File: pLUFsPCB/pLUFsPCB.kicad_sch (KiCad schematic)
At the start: 9 parts, among them J1 Circular Display Pins (R), J2 Circular Display Pins (L), M1 Stepper_Motor_bipolar, SW2 BT Button, U1 ESP32 C3, U2 TB6612FNG

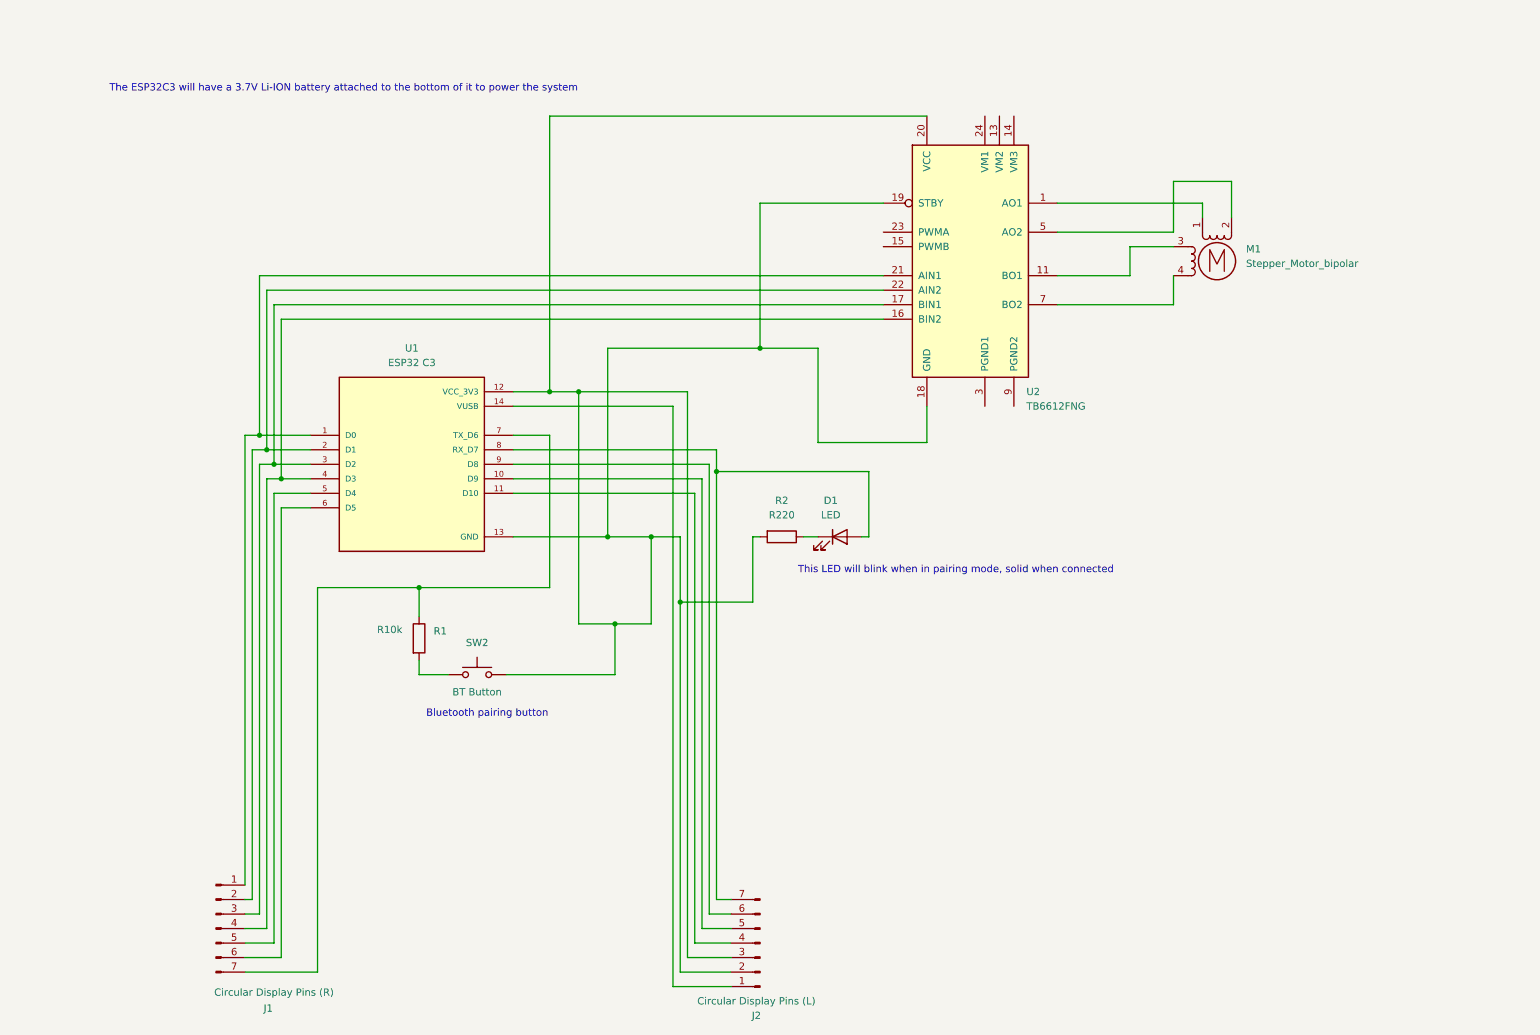
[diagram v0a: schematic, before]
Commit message: lots
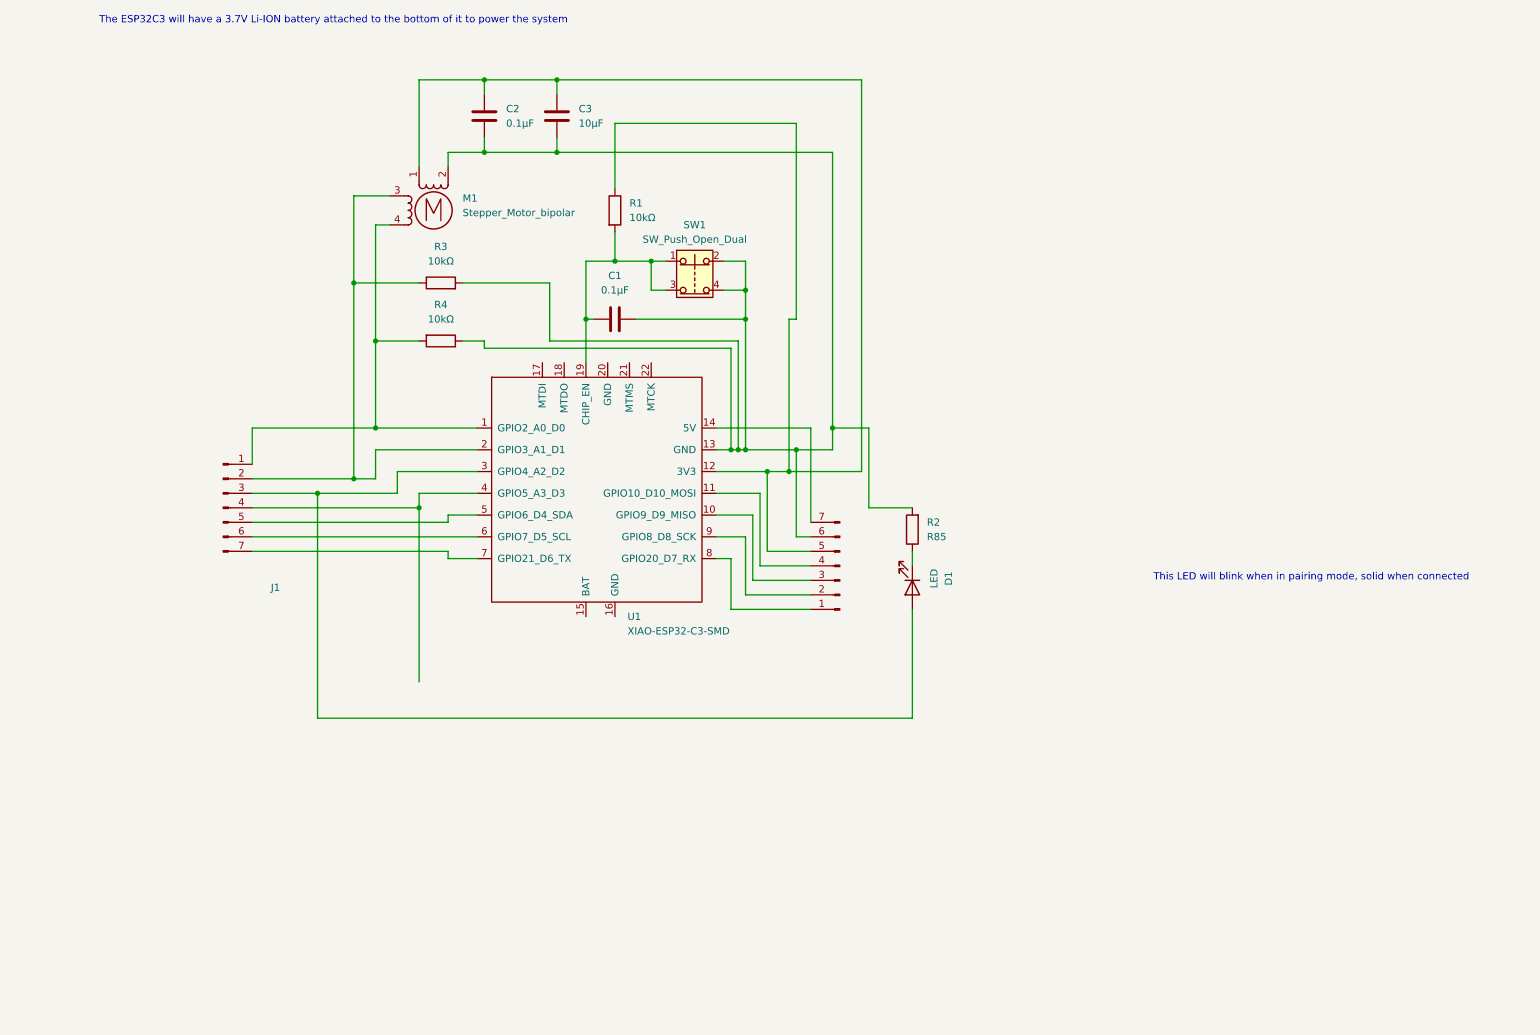
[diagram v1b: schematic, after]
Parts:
- removed SW2: BT Button, symbol Switch:SW_Push
- removed U1: ESP32 C3, 113991054:MODULE_113991054, symbol 113991054:113991054
- removed U2: TB6612FNG, Package_SO:SSOP-24_5.3x8.2mm_P0.65mm, symbol Driver_Motor:TB6612FNG
- added C1, C2: 0.1μF, Capacitor_SMD:C_0805_2012Metric, symbol Device:C
- added C3: 10μF, Capacitor_SMD:C_0805_2012Metric, symbol Device:C
- added R3, R4: 10kΩ, Resistor_SMD:R_0805_2012Metric, symbol Device:R
- added SW1: SW_Push_Open_Dual, Button_Switch_SMD:SW_MEC_5GSH9, symbol Switch:SW_Push_Open_Dual
- added U1: XIAO-ESP32-C3-SMD, RF_Module:MCU_Seeed_ESP32C3, symbol Seeed_Studio_XIAO_Series:XIAO-ESP32-C3-SMD
- D1: footprint (none) -> LED_SMD:LED_0603_1608Metric
- J1: value Circular Display Pins (R) -> Circular Display Pins (bottom); footprint (none) -> Connector_PinHeader_2.54mm:PinHeader_1x07_P2.54mm_Vertical
- J2: value Circular Display Pins (L) -> Circular Display Pins (top); footprint (none) -> Connector_PinHeader_2.54mm:PinHeader_1x07_P2.54mm_Vertical
- M1: footprint (none) -> Stepper Footprint:x27_stepper
- R1: value R10k -> 10kΩ; footprint (none) -> Resistor_SMD:R_0805_2012Metric
- R2: value R220 -> R85; footprint (none) -> Resistor_SMD:R_0805_2012Metric
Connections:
- net at R1.2: now also C1.2, SW1.1, SW1.3, U1.19 (CHIP_EN)
- net at R1.1: now also J2.5 (Pin_5), M1.1, C2.1, C3.1, U1.12 (3V3); no longer J1.7 (Pin_7)
- net at J1.1 (Pin_1): now also M1.4, R4.2, U1.1 (GPIO2_A0_D0)
- net at J2.4 (Pin_4): now also U1.11 (GPIO10_D10_MOSI)
- net at J2.1 (Pin_1): now also U1.8 (GPIO20_D7_RX)
- net at J1.2 (Pin_2): now also M1.3, R3.1, U1.2 (GPIO3_A1_D1)
- net at J1.3 (Pin_3): now also D1.2 (A), U1.3 (GPIO4_A2_D2)
- net at J1.4 (Pin_4): now also U1.4 (GPIO5_A3_D3)
- net at J1.5 (Pin_5): now also U1.5 (GPIO6_D4_SDA)
- net at J1.6 (Pin_6): now also U1.6 (GPIO7_D5_SCL)
- net at J2.7 (Pin_7): now also U1.14 (5V); no longer D1.2 (A)
- net at J2.6 (Pin_6): now also M1.2 (-), R2.2, C1.1, C2.2, C3.2, R3.2, R4.1, SW1.2, SW1.4, U1.13 (GND)
- new net: J2.3 (Pin_3), U1.10 (GPIO9_D9_MISO)
- new net: J1.7 (Pin_7), U1.7 (GPIO21_D6_TX)
- new net: J2.2 (Pin_2), U1.9 (GPIO8_D8_SCK)
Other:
- note removed: "Bluetooth pairing button"
- title: (none) -> pLUFs Schematic; Second Draft
- moved on the sheet: D1, R2
